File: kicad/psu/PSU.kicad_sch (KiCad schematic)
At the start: 47 parts, among them J1 B2B-PH-K-S, J2 Conn_01x07_Pin, U1 BQ21040DBVR, U2 RT4812GJ8F, U3 AP3445LW6-7, U4 AP3445LW6-7

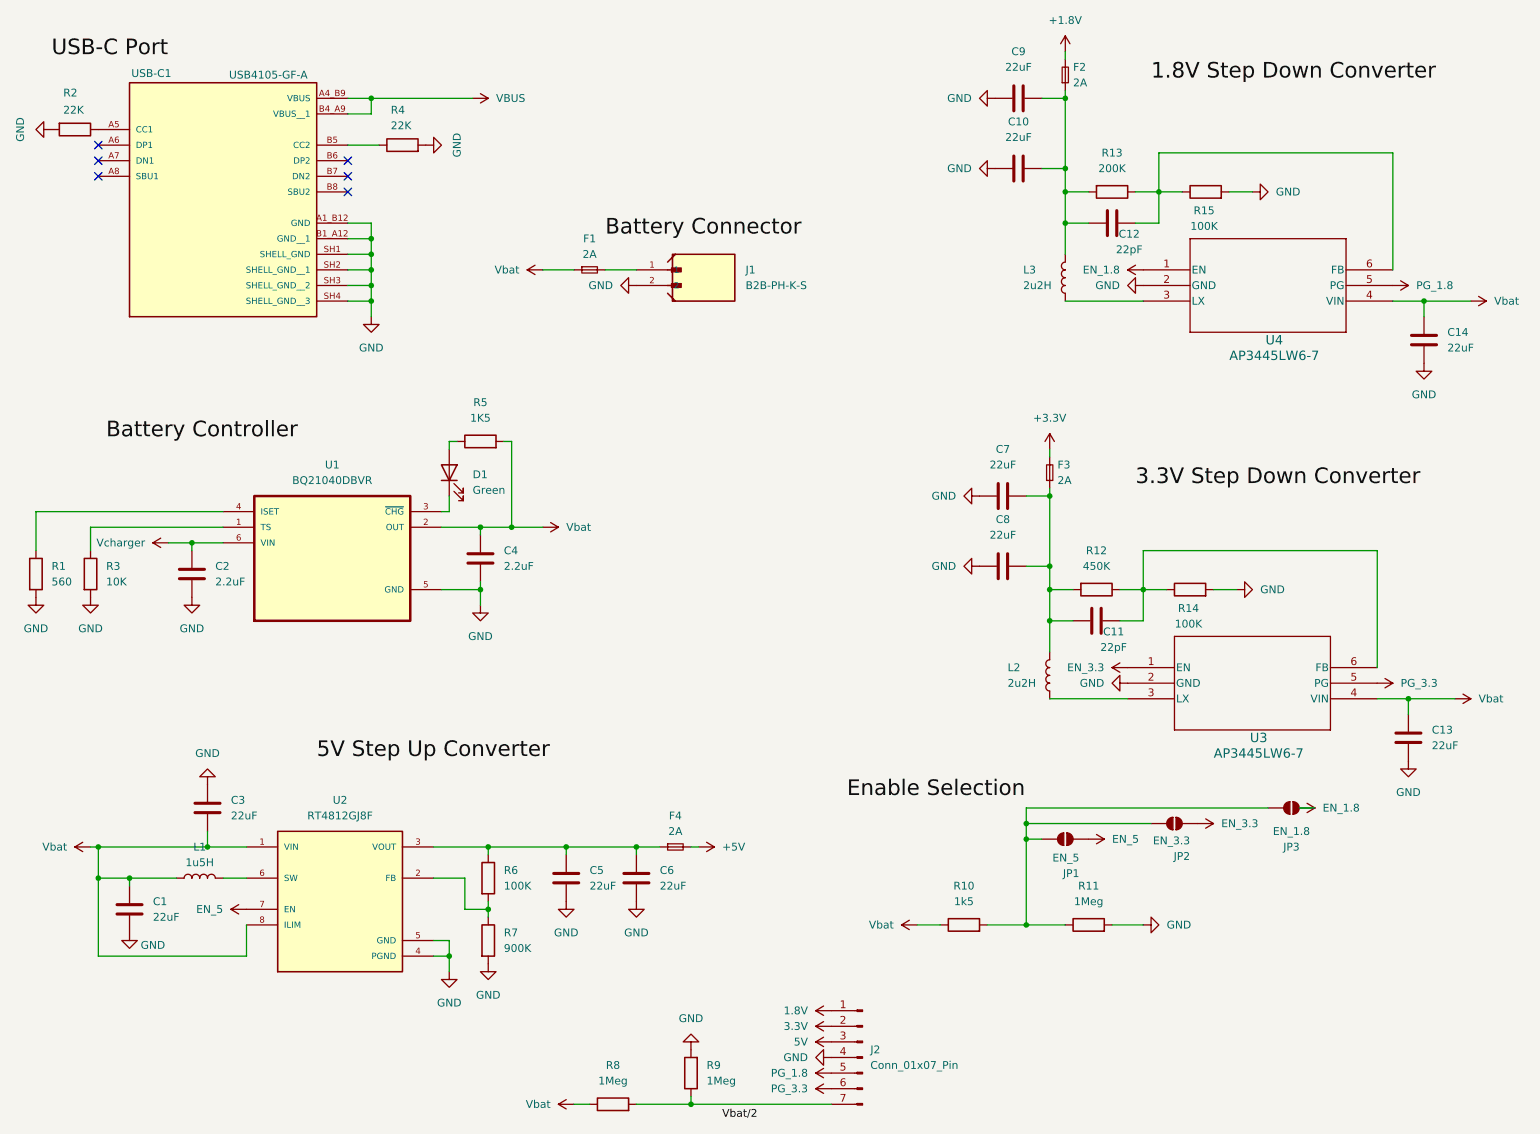
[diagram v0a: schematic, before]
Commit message: Update PSU.kicad_sch
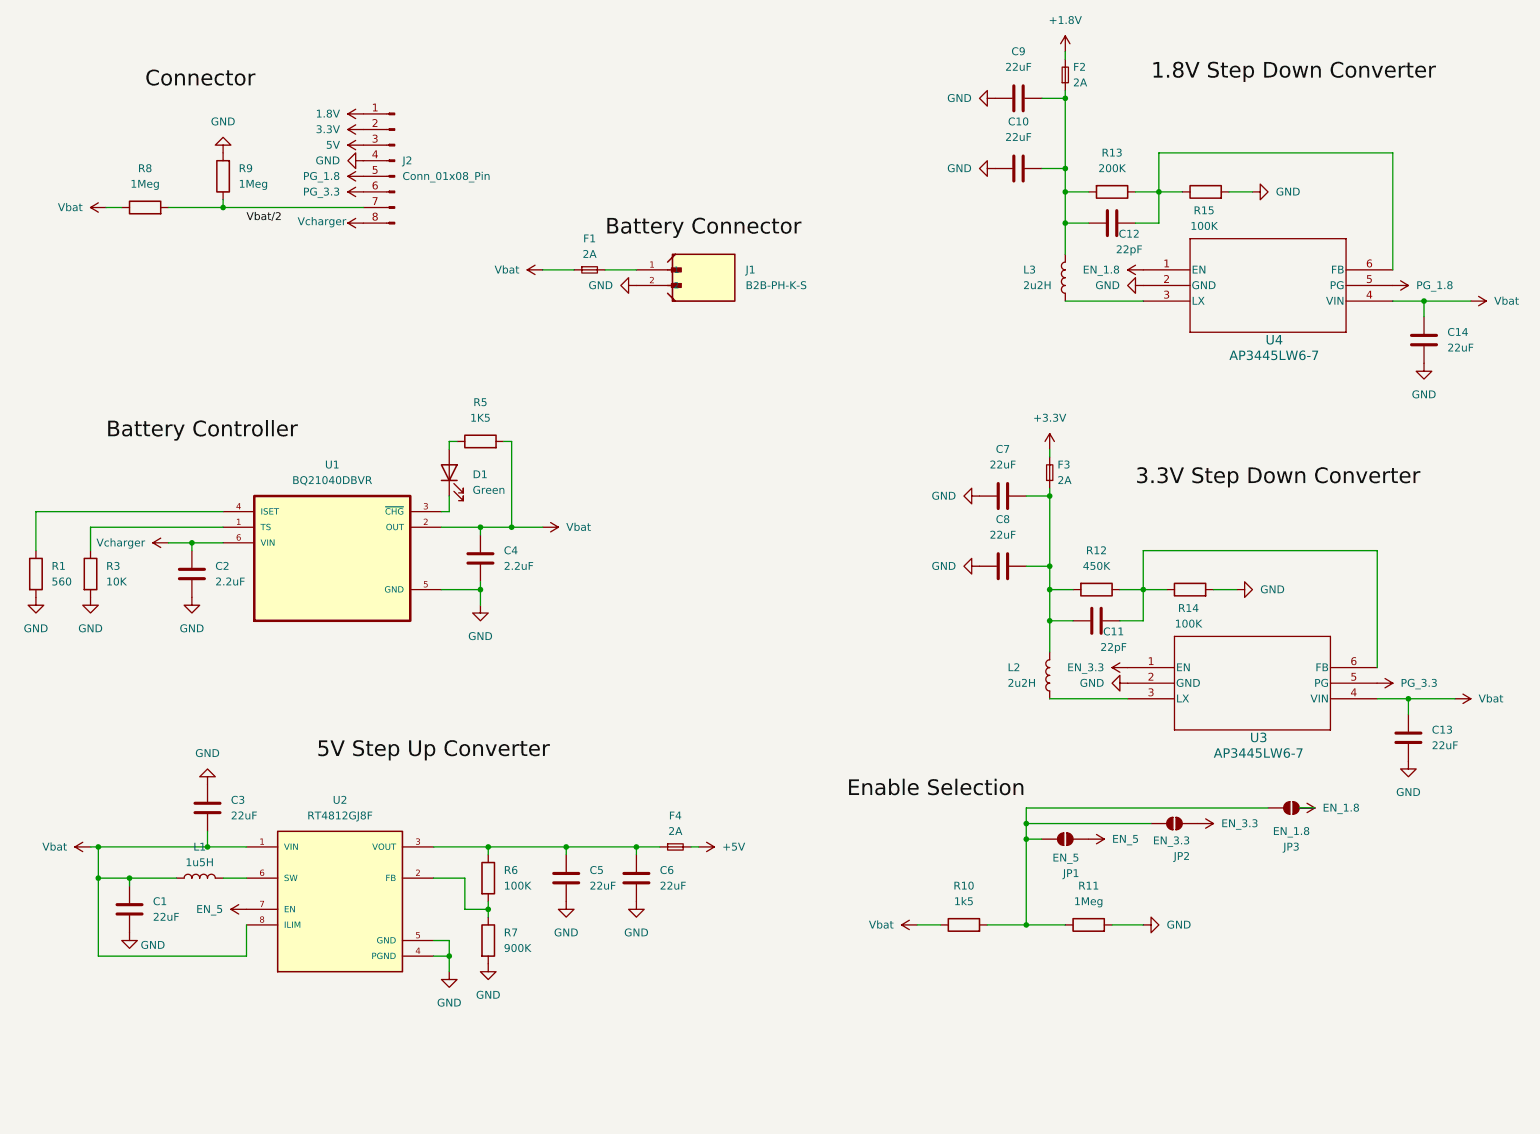
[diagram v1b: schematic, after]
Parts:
- removed J2: Conn_01x07_Pin, symbol Connector:Conn_01x07_Pin
- removed R2, R4: 22K, Resistor_SMD:R_0805_2012Metric, symbol Device:R
- removed USB-C1: USB4105-GF-A, USB4105-GF-A-120:GCT_USB4105-GF-A-120, symbol USB4105-GF-A-120:USB4105-GF-A-120
- added J2: Conn_01x08_Pin, symbol Connector:Conn_01x08_Pin
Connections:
- net 1.8V: now also J2.1 (Pin_1)
- net 3.3V: now also J2.2 (Pin_2)
- net 5V: now also J2.3 (Pin_3)
- net GND: now also J2.4 (Pin_4)
- net PG_1.8: now also J2.5 (Pin_5)
- net PG_3.3: now also J2.6 (Pin_6)
- net Vcharger: now also J2.8 (Pin_8)
- net at R8.2, R9.1: now also J2.7 (Pin_7)
- no-connect marks 6 -> 0
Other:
- moved on the sheet: R8, R9
